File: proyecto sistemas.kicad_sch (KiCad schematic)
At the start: 0 parts

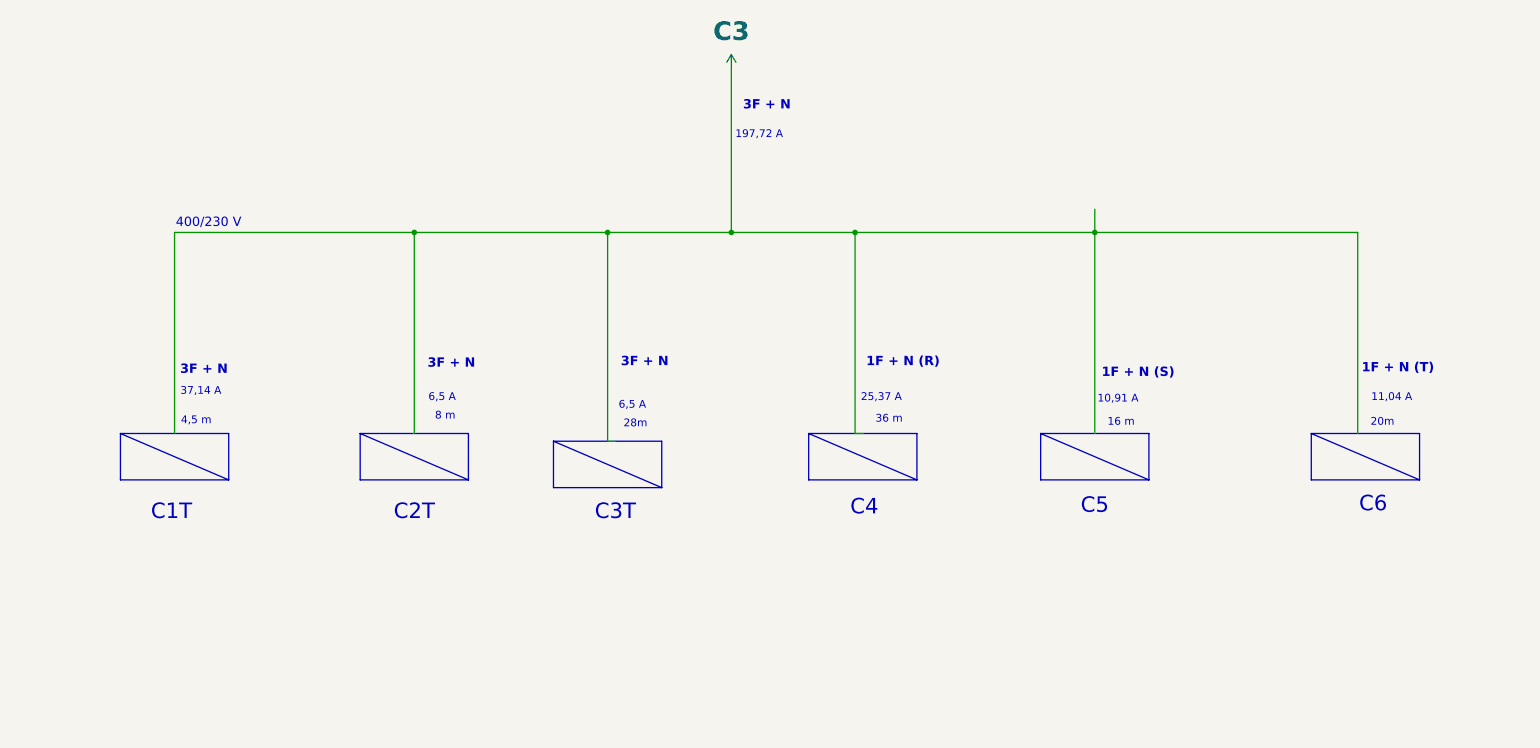
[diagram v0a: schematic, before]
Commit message: unifilar nuevo 10/13/2025
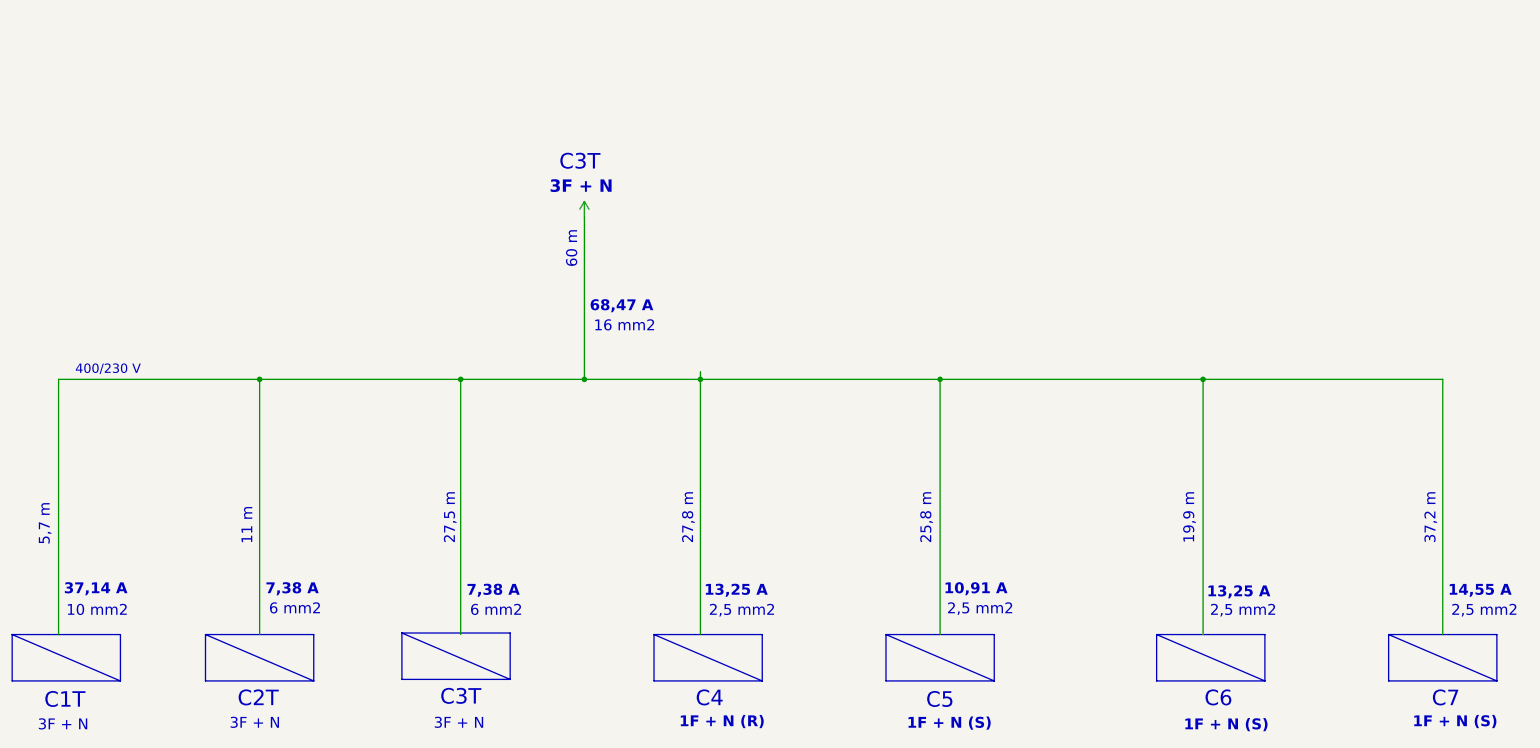
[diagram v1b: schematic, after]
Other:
- note added: "10 mm2"
- note added: "11 m"
- note added: "13,25 A"
- note added: "14,55 A"
- note added: "16 mm2"
- note added: "19,9 m"
- note added: "2,5 mm2"
- note added: "25,8 m"
- note added: "27,5 m"
- note added: "27,8 m"
- note added: "37,2 m"
- note added: "5,7 m"
- note added: "6 mm2"
- note added: "60 m"
- note added: "68,47 A"
- note added: "7,38 A"
- note added: "C7"
- note removed: "11,04 A"
- note removed: "16 m"
- note removed: "197,72 A"
- note removed: "1F + N (T)"
- note removed: "20m"
- note removed: "25,37 A"
- note removed: "28m"
- note removed: "36 m"
- note removed: "4,5 m"
- note removed: "6,5 A"
- note removed: "8 m"
